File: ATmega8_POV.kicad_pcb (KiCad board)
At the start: 2 copper layers, 17.2 x 154.5 mm, 23 parts, among them IC1 ATMEGA8-P, P1 CONN_01X02, Y1 Crystal_Small

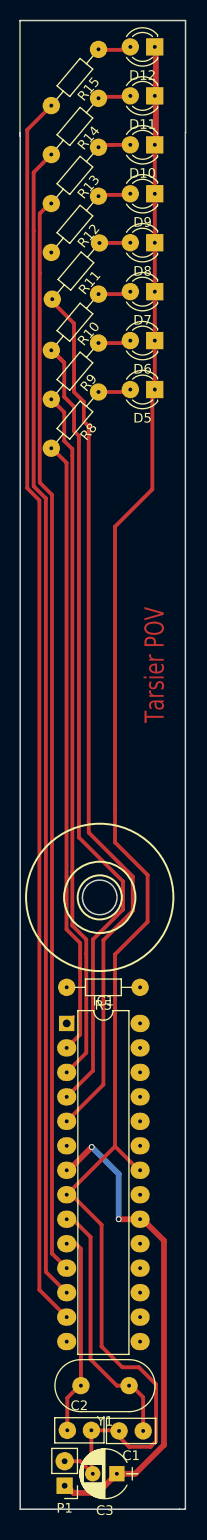
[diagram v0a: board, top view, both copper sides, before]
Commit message: *changing footprints
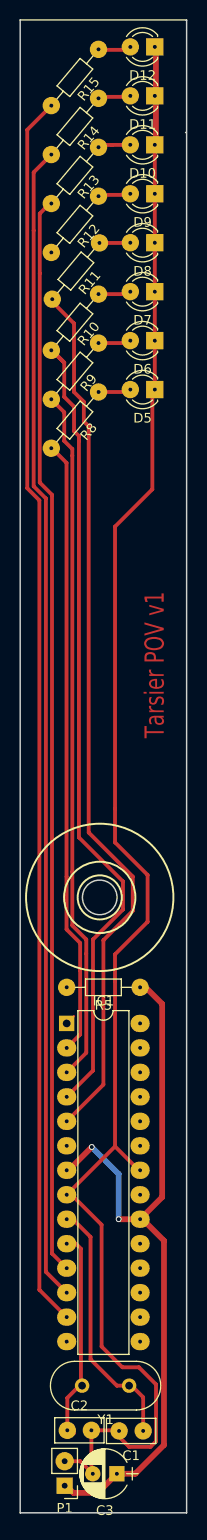
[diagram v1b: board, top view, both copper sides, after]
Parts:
- Y1: footprint Crystals:Resonator-2pin_w10.0mm_h5.0mm -> Crystals:Crystal_HC49-4H_Vertical
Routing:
- net VCC: track 51.8 -> 78.1 mm
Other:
- board size 17.2 x 154.5 mm -> 17.3 x 154.9 mm
- board text added: "Tarsier POV v1"
- board text removed: "Tarsier POV"
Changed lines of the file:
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@@
   (general
     (links 38)
-    (no_connects 3)
-    (area 88.804679 39.096879 106.145401 193.750001)
+    (no_connects 2)
+    (area 88.824999 39.040999 106.247001 194.131001)
     (thickness 1.6)
-    (drawings 13)
-    (tracks 171)
+    (drawings 12)
+    (tracks 175)
     (zones 0)
     (modules 23)
@@
   )
   (setup
-    (last_trace_width 0.4)
+    (last_trace_width 0.6)
     (user_trace_width 0.4)
     (user_trace_width 0.6)
@@
     (add_net "Net-(IC1-Pad1)")
     (add_net VCC)
-  )
-  (module Crystals:Resonator-2pin_w10.0mm_h5.0mm (layer F.Cu)
-    (at 100.203 180.848 180)
-    (descr "Ceramic Resomator/Filter 10.0x5.0 RedFrequency MG/MT/MX series, http://www.red-frequency.com/download/datenblatt/redfrequency-datenblatt-ir-zta.pdf, length*width=10.0x5.0mm^2 package, package length=10.0mm, package width=5.0mm, 2 pins")
-    (tags "THT ceramic resonator filter")
-    (fp_text reference Y1 (at 2.5 -3.7 180) (layer F.SilkS)
-      (effects (font (size 1 1) (thickness 0.15)))
-    )
-    (fp_text value Crystal_Small (at 2.5 3.7 180) (layer F.Fab)
-      (effects (font (size 1 1) (thickness 0.15)))
-    )
-    (fp_text user %R (at 2.54 0 180) (layer F.Fab)
-      (effects (font (size 1 1) (thickness 0.15)))
-    )
-    (fp_line (start 0 -2.5) (end 5 -2.5) (layer F.Fab) (width 0.1))
-    (fp_line (start 0 2.5) (end 5 2.5) (layer F.Fab) (width 0.1))
-    (fp_line (start 0 -2.5) (end 5 -2.5) (layer F.Fab) (width 0.1))
-    (fp_line (start 0 2.5) (end 5 2.5) (layer F.Fab) (width 0.1))
-    (fp_line (start 0 -2.7) (end 5 -2.7) (layer F.SilkS) (width 0.12))
-    (fp_line (start 0 2.7) (end 5 2.7) (layer F.SilkS) (width 0.12))
-    (fp_line (start -3 -3) (end -3 3) (layer F.CrtYd) (width 0.05))
-    (fp_line (start -3 3) (end 8 3) (layer F.CrtYd) (width 0.05))
-    (fp_line (start 8 3) (end 8 -3) (layer F.CrtYd) (width 0.05))
-    (fp_line (start 8 -3) (end -3 -3) (layer F.CrtYd) (width 0.05))
-    (fp_arc (start 0 0) (end 0 -2.5) (angle -180) (layer F.Fab) (width 0.1))
-    (fp_arc (start 5 0) (end 5 -2.5) (angle 180) (layer F.Fab) (width 0.1))
-    (fp_arc (start 0 0) (end 0 -2.5) (angle -180) (layer F.Fab) (width 0.1))
-    (fp_arc (start 5 0) (end 5 -2.5) (angle 180) (layer F.Fab) (width 0.1))
-    (fp_arc (start 0 0) (end 0 -2.7) (angle -180) (layer F.SilkS) (width 0.12))
-    (fp_arc (start 5 0) (end 5 -2.7) (angle 180) (layer F.SilkS) (width 0.12))
-    (pad 1 thru_hole circle (at 0 0 180) (size 1.8 1.8) (drill 0.4) (layers *.Cu *.Mask)
-      (net 1 "Net-(C1-Pad1)"))
-    (pad 2 thru_hole circle (at 5 0 180) (size 1.8 1.8) (drill 0.4) (layers *.Cu *.Mask)
-      (net 3 "Net-(C2-Pad1)"))
-    (model ${KISYS3DMOD}/Crystals.3dshapes/Resonator-2pin_w10.0mm_h5.0mm.wrl
-      (at (xyz 0 0 0))
-      (scale (xyz 0.393701 0.393701 0.393701))
-      (rotate (xyz 0 0 0))
-    )
   )
   (module Housings_DIP:DIP-28_W7.62mm (layer F.Cu)
@@
     )
   )
-  (gr_line (start 88.87968 39.17188) (end 106.06024 39.17188) (angle 90) (layer Edge.Cuts) (width 0.15))
+  (module Crystals:Crystal_HC49-4H_Vertical (layer F.Cu)
+    (at 100.203 180.848 180)
+    (descr "Crystal THT HC-49-4H http://5hertz.com/pdfs/04404_D.pdf")
+    (tags "THT crystalHC-49-4H")
+    (fp_text reference Y1 (at 2.44 -3.525 180) (layer F.SilkS)
+      (effects (font (size 1 1) (thickness 0.15)))
+    )
+    (fp_text value Crystal_Small (at 2.44 3.525 180) (layer F.Fab)
+      (effects (font (size 1 1) (thickness 0.15)))
+    )
+    (fp_text user %R (at 2.44 0 180) (layer F.Fab)
+      (effects (font (size 1 1) (thickness 0.15)))
+    )
+    (fp_line (start -0.76 -2.325) (end 5.64 -2.325) (layer F.Fab) (width 0.1))
+    (fp_line (start -0.76 2.325) (end 5.64 2.325) (layer F.Fab) (width 0.1))
+    (fp_line (start -0.56 -2) (end 5.44 -2) (layer F.Fab) (width 0.1))
+    (fp_line (start -0.56 2) (end 5.44 2) (layer F.Fab) (width 0.1))
+    (fp_line (start -0.76 -2.525) (end 5.64 -2.525) (layer F.SilkS) (width 0.12))
+    (fp_line (start -0.76 2.525) (end 5.64 2.525) (layer F.SilkS) (width 0.12))
+    (fp_line (start -3.6 -2.8) (end -3.6 2.8) (layer F.CrtYd) (width 0.05))
+    (fp_line (start -3.6 2.8) (end 8.5 2.8) (layer F.CrtYd) (width 0.05))
+    (fp_line (start 8.5 2.8) (end 8.5 -2.8) (layer F.CrtYd) (width 0.05))
+    (fp_line (start 8.5 -2.8) (end -3.6 -2.8) (layer F.CrtYd) (width 0.05))
+    (fp_arc (start -0.76 0) (end -0.76 -2.325) (angle -180) (layer F.Fab) (width 0.1))
+    (fp_arc (start 5.64 0) (end 5.64 -2.325) (angle 180) (layer F.Fab) (width 0.1))
+    (fp_arc (start -0.56 0) (end -0.56 -2) (angle -180) (layer F.Fab) (width 0.1))
+    (fp_arc (start 5.44 0) (end 5.44 -2) (angle 180) (layer F.Fab) (width 0.1))
+    (fp_arc (start -0.76 0) (end -0.76 -2.525) (angle -180) (layer F.SilkS) (width 0.12))
+    (fp_arc (start 5.64 0) (end 5.64 -2.525) (angle 180) (layer F.SilkS) (width 0.12))
+    (pad 1 thru_hole circle (at 0 0 180) (size 1.5 1.5) (drill 0.8) (layers *.Cu *.Mask)
+      (net 1 "Net-(C1-Pad1)"))
+    (pad 2 thru_hole circle (at 4.88 0 180) (size 1.5 1.5) (drill 0.8) (layers *.Cu *.Mask)
+      (net 3 "Net-(C2-Pad1)"))
+    (model ${KISYS3DMOD}/Crystals.3dshapes/Crystal_HC49-4H_Vertical.wrl
+      (at (xyz 0 0 0))
+      (scale (xyz 0.393701 0.393701 0.393701))
+      (rotate (xyz 0 0 0))
+    )
+  )
+  (gr_line (start 106.172 194.056) (end 106.172 39.116) (angle 90) (layer Edge.Cuts) (width 0.15))
+  (gr_line (start 88.9 194.056) (end 106.172 194.056) (angle 90) (layer Edge.Cuts) (width 0.15))
+  (gr_line (start 88.9 39.116) (end 88.9 194.056) (angle 90) (layer Edge.Cuts) (width 0.15))
+  (gr_line (start 106.172 39.116) (end 88.9 39.116) (angle 90) (layer Edge.Cuts) (width 0.15))
+  (dimension 154.432 (width 0.3) (layer Eco2.User)
+    (gr_text "154.432 mm" (at 109.553999 116.332 270) (layer Eco2.User)
+      (effects (font (size 1.5 1.5) (thickness 0.3)))
+    )
+    (feature1 (pts (xy 106.172 193.548) (xy 110.903999 193.548)))
+    (feature2 (pts (xy 106.172 39.116) (xy 110.903999 39.116)))
+    (crossbar (pts (xy 108.203999 39.116) (xy 108.203999 193.548)))
+    (arrow1a (pts (xy 108.203999 193.548) (xy 107.617578 192.421496)))
+    (arrow1b (pts (xy 108.203999 193.548) (xy 108.79042 192.421496)))
+    (arrow2a (pts (xy 108.203999 39.116) (xy 107.617578 40.242504)))
+    (arrow2b (pts (xy 108.203999 39.116) (xy 108.79042 40.242504)))
+  )
+  (dimension 17.272 (width 0.3) (layer Eco2.User)
+    (gr_text "17.272 mm" (at 97.536 34.718) (layer Eco2.User)
+      (effects (font (size 1.5 1.5) (thickness 0.3)))
+    )
+    (feature1 (pts (xy 106.172 38.608) (xy 106.172 33.368)))
+    (feature2 (pts (xy 88.9 38.608) (xy 88.9 33.368)))
+    (crossbar (pts (xy 88.9 36.068) (xy 106.172 36.068)))
+    (arrow1a (pts (xy 106.172 36.068) (xy 105.045496 36.654421)))
+    (arrow1b (pts (xy 106.172 36.068) (xy 105.045496 35.481579)))
+    (arrow2a (pts (xy 88.9 36.068) (xy 90.026504 36.654421)))
+    (arrow2b (pts (xy 88.9 36.068) (xy 90.026504 35.481579)))
+  )
   (gr_line (start 106.06024 50.8) (end 106.0704 50.78984) (angle 90) (layer Edge.Cuts) (width 0.15))
-  (gr_line (start 106.06024 39.17188) (end 106.06024 50.8) (angle 90) (layer Edge.Cuts) (width 0.15))
-  (gr_line (start 88.87968 51.14544) (end 88.87968 39.17188) (angle 90) (layer Edge.Cuts) (width 0.15))
-  (gr_text "Tarsier POV" (at 102.87 106.045 90) (layer F.Cu)
+  (gr_text "Tarsier POV v1" (at 102.87 106.045 90) (layer F.Cu)
     (effects (font (size 2 1.5) (thickness 0.375)))
   )
@@
   (gr_circle (center 97.155 130.175) (end 98.425 131.445) (layer Edge.Cuts) (width 0.15))
   (gr_circle (center 97.155 130.175) (end 99.06 133.35) (layer F.SilkS) (width 0.2))
-  (gr_line (start 106.045 193.675) (end 106.045 50.8) (angle 90) (layer Edge.Cuts) (width 0.15))
-  (gr_line (start 105.41 193.675) (end 106.045 193.675) (angle 90) (layer Edge.Cuts) (width 0.15))
-  (gr_line (start 88.9 193.675) (end 105.41 193.675) (angle 90) (layer Edge.Cuts) (width 0.15))
-  (gr_line (start 88.9 50.8) (end 88.9 193.675) (angle 90) (layer Edge.Cuts) (width 0.15))
   (segment (start 101.346 171.196) (end 100.98024 171.196) (width 0.25) (layer F.Cu) (net 0))
   (segment (start 101.346 171.196) (end 101.28758 171.196) (width 0.25) (layer F.Cu) (net 0))
@@
   (segment (start 94.2359 185.77814) (end 94.29814 185.77814) (width 0.4) (layer F.Cu) (net 3))
   (segment (start 94.2359 185.77814) (end 94.47276 185.77814) (width 0.25) (layer F.Cu) (net 3))
+  (segment (start 101.346 139.5095) (end 101.9175 139.5095) (width 0.25) (layer F.Cu) (net 4) (status C00000))
+  (segment (start 101.9175 139.5095) (end 103.632 141.224) (width 0.6) (layer F.Cu) (net 4) (status 400000))
+  (segment (start 103.632 161.29) (end 101.346 163.576) (width 0.6) (layer F.Cu) (net 4) (status 800000))
+  (segment (start 103.632 141.224) (end 103.632 161.29) (width 0.6) (layer F.Cu) (net 4))
   (segment (start 93.51264 191.23152) (end 93.6752 191.23152) (width 0.6) (layer F.Cu) (net 4))
   (segment (start 93.6752 191.23152) (end 94.42196 191.97828) (width 0.6) (layer F.Cu) (net 4))
